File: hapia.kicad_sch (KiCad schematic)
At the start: 63 parts, among them CN1 100nf, CN2 100nf, J1 Conn_ARM_JTAG_SWD_10, J2 USB_C_Receptacle_USB2.0_16P, SW1 SW_Push, SW2 SW_Push, U1 STM32F407VET6, U11 SRV05-4HTG-D, U2 AMS1117-3.3, Y1 8mhz

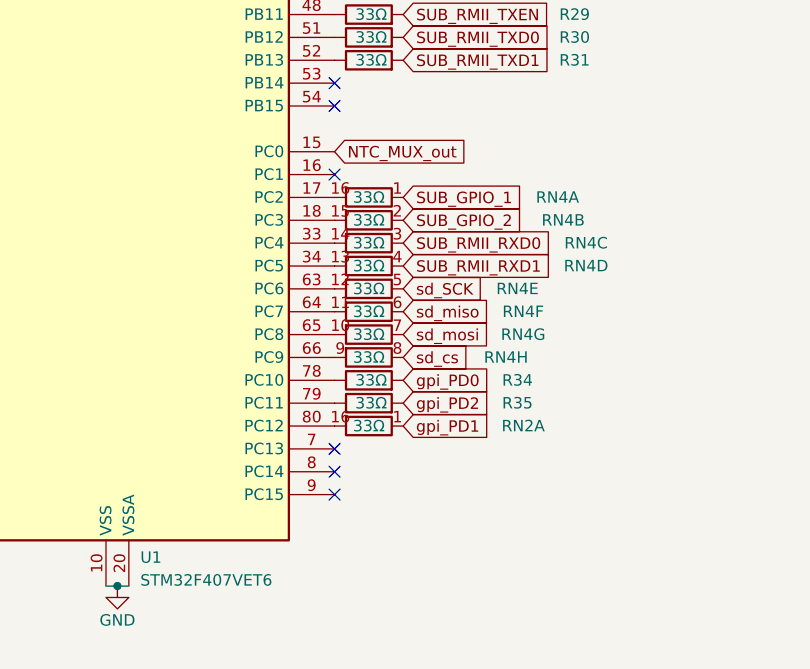
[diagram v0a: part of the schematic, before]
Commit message: 27092026/0002
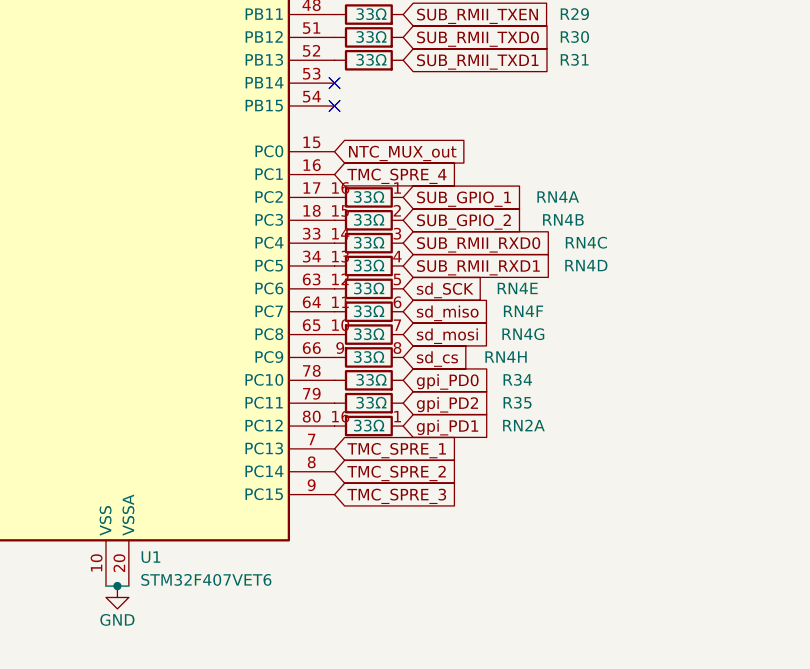
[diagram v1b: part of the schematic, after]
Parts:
- D2: footprint (none) -> LED_THT:LED_D3.0mm_FlatTop; jlc_pcb: (none) -> C7148823; mouser: (none) -> 78-VLCS5130; mpn (none) -> VLCS5130
- R1, R27: footprint (none) -> Resistor_SMD:R_0603_1608Metric Resistor_SMD_R_0603_1608Metric; jlc_pcb: (none) -> C13564; mouser: (none) -> 81-NCP18XH103F03RB; mpn (none) -> NCP18XH103F03RB
- R48: footprint (none) -> Capacitor_SMD:C_0603_1608Metric_Pad1.08x0.95mm_HandSolder; jlc_pcb: (none) -> C22548; mouser: (none) -> 603-RC0603FR-071KL; mpn (none) -> RC0603FR-071KL
- R50, R51: footprint Resistor_SMD:R_0603_1608Metric Resistor_SMD:R_0603_1608Metric -> Resistor_SMD:R_0603_1608Metric Resistor_SMD_R_0603_1608Metric
- R52: footprint (none) -> Resistor_SMD:R_0805_2012Metric_Pad1.20x1.40mm_HandSolder; jlc_pcb: (none) -> C114564; mouser: (none) -> 603-RC0805FR-07470RL; mpn (none) -> RC0805FR-07470RL
- R53, R54: footprint (none) -> Capacitor_SMD:C_0402_1005Metric_Pad0.74x0.62mm_HandSolder
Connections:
- net TMC_SPRE_4: now reaches U1.16 (PC1)
- net TMC_SPRE_1: now reaches U1.7 (PC13)
- net TMC_SPRE_2: now reaches U1.8 (PC14)
- net TMC_SPRE_3: now reaches U1.9 (PC15)
- no-connect marks 20 -> 16

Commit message: sch antigo tava jogado no pc
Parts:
- removed C6: 10µf, Capacitor_SMD:C_1206_3216Metric_Pad1.33x1.80mm_HandSolder, symbol Device:C
- removed C84: 100nf, Capacitor_SMD:C_0603_1608Metric, symbol Device:C
- removed CN1, CN2: 100nf, Capacitor_SMD:C_0603_1608Metric, symbol Device:C_Network04
- removed D2: RED, LED_THT:LED_D3.0mm_FlatTop, symbol Device:LED_Small
- removed D9: SMF3.3, Diode_SMD:D_SMF, symbol Diode:SMF5V0A
- removed F1: Fuse, symbol Device:Fuse
- removed J1: Conn_ARM_JTAG_SWD_10, symbol Connector:Conn_ARM_JTAG_SWD_10
- removed J2: USB_C_Receptacle_USB2.0_16P, Connector_USB:USB_C_Receptacle_HCTL_HC-TYPE-C-16P-01A, symbol Connector:USB_C_Receptacle_USB2.0_16P
- removed JP1: usb/atx, Jumper:SolderJumper-3_P1.3mm_Bridged2Bar12_RoundedPad1.0x1.5mm, symbol Jumper:SolderJumper_3_Bridged12
- removed R110, R111, R112, R113, R41, R42, R75: 33Ω, Resistor_SMD:R_0603_1608Metric_Pad0.98x0.95mm_HandSolder, symbol Device:R
- removed R52: 470Ω, Resistor_SMD:R_0805_2012Metric_Pad1.20x1.40mm_HandSolder, symbol Device:R_Small
- removed R54: 5.1kΩ, Capacitor_SMD:C_0402_1005Metric_Pad0.74x0.62mm_HandSolder, symbol Device:R
- removed RN2, RN4: 33Ω, Resistor_SMD:R_0603_1608Metric_Pad0.98x0.95mm_HandSolder, symbol Device:R_Pack08_Split
- removed RN5: 33Ω, Resistor_SMD:R_0603_1608Metric_Pad0.98x0.95mm_HandSolder, symbol Device:R_Pack04_Split
- removed TP1: TestPoint, TestPoint:TestPoint_Pad_D1.0mm, symbol Connector:TestPoint
- removed U11: SRV05-4HTG-D, Package_TO_SOT_SMD:SOT-23-6, symbol Power_Protection:SRV05-4
- removed U2: AMS1117-3.3, Package_TO_SOT_SMD:SOT-223-3_TabPin2, symbol Regulator_Linear:AMS1117-3.3
- added C1, C2, C21, C28, C43, C45, C59: 4.7uf, symbol Device:C
- added C13, C14, C16, C20, C23, C24, C26, C29, C34, C35, C36, C37, C39, C41, C46, C48, C53, C54, C55, C56, C58, C61, C63, C64, C65, C66, C68, C69, C70, C71: 100nf, symbol Device:C
- added C15, C25, C38, C40, C57, C62: 1uf, symbol Device:C
- added C17, C32, C33: 22nf, symbol Device:C
- added C18, C30, C47, C49, C67, C73: 10uf, symbol Device:C
- added C19, C31, C50, C51: 100uf, symbol Device:C
- added C22, C27, C42, C44, C74: 10nf, symbol Device:C
- added C52, C60: 1000uf, symbol Device:C
- added D1: D_Schottky, symbol Device:D_Schottky
- added F1, F3, F4: Polyfuse, symbol Device:Polyfuse
- added F2: Fuse, symbol Device:Fuse
- added FB2: FerriteBead, symbol Device:FerriteBead
- added J1: ATX-20, Connector_Molex:Molex_Mini-Fit_Jr_5566-20A_2x10_P4.20mm_Vertical, symbol Connector:ATX-20
- added J2: Micro_SD_Card, symbol Connector:Micro_SD_Card
- added J3, J4, J5, J6: Conn_01x04_Pin, Connector_JST:JST_EH_B4B-EH-A_1x04_P2.50mm_Vertical, symbol Connector:Conn_01x04_Pin
- added J7: Conn_01x15_Pin, Connector_PinSocket_2.54mm:PinSocket_1x15_P2.54mm_Vertical, symbol Connector:Conn_01x15_Pin
- added L1: 6.8uh, Inductor_SMD:L_Bourns_SRP1038C_10.0x10.0mm, symbol Device:L
- added M1: Fan, symbol Motor:Fan
- added Q1, Q3: NMOS, symbol Simulation_SPICE:NMOS
- added R10, R11, R12, R13, R17, R18, R19, R20, R3: 100k, symbol Device:R
- added R14, R21, R22, R9: 20k, symbol Device:R
- added R15, R16, R23, R24, R5, R6: 11r, symbol Device:R
- added R2: 10K, symbol Device:R
- added R37: 10k, symbol Device:R
- added R38: 330r, symbol Device:R
- added R39: 100r, symbol Device:R
- added R4: 22k, symbol Device:R
- added R41: exrtusora, symbol Device:Heater
- added R43, R45, R46, R47, R48, R52, R8: 33r, symbol Device:R
- added SW3: SW_Push, symbol Switch:SW_Push
- added TP3: TestPoint, Connector_USB:USB_Micro-B_Amphenol_10104110_Horizontal, symbol Connector:TestPoint
- added U2, U4, U5, U6: TMC2209-LA, Package_DFN_QFN:VQFN-28-1EP_5x5mm_P0.5mm_EP3.7x3.7mm_ThermalVias, symbol Driver_Motor:TMC2209-LA
- added U3: TPS54302, Package_TO_SOT_SMD:SOT-23-6, symbol Regulator_Switching:TPS54302
- C10: value 4.7µf -> 100nf; footprint Capacitor_SMD:C_0603_1608Metric_Pad1.08x0.95mm_HandSolder -> (none); jlc_pcb: C162274 -> (none); mouser: 81-GRM188R61E475KE1D -> (none); mpn GRM188R61E475KE11D -> (none)
- C11: value 10µf -> 100nf; footprint Capacitor_SMD:C_1206_3216Metric_Pad1.33x1.80mm_HandSolder -> (none); jlc_pcb: C13585 -> (none); mouser: 187-CL31B106KLK6PNE -> (none); mpn CL31A106KBHNNNE -> (none)
- C12: value 1µf -> 22nf; footprint Capacitor_SMD:C_0805_2012Metric_Pad1.18x1.45mm_HandSolder -> (none); jlc_pcb: C28323 -> (none); mouser: 187-CL21B105KBFNNNE -> (none); mpn CL21B105KBFNNNE -> (none)
- C3: renamed from C5; value 22pf -> pf; footprint Capacitor_SMD:C_0603_1608Metric_Pad1.08x0.95mm_HandSolder -> (none); jlc_pcb: C561800 -> (none); mouser: 80-C0603C220J4G -> (none); mpn C0603C220J4GAC7867 -> (none)
- C4: renamed from C1; value 22pf -> pf; footprint Capacitor_SMD:C_0603_1608Metric_Pad1.08x0.95mm_HandSolder -> (none); jlc_pcb: C561800 -> (none); mouser: 80-C0603C220J4G -> (none); mpn C0603C220J4GAC7867 -> (none)
- C5: renamed from C4; footprint Capacitor_SMD:C_0603_1608Metric -> (none); jlc_pcb/lcsc_ID: C346191 -> (none); jlc_pcb: C307348 -> (none); mouser: 187-CL10B104KB8WPNC -> (none); mpn CL10B104KB8WPNC -> (none)
- C6: renamed from C3; footprint Capacitor_SMD:C_0603_1608Metric -> (none); jlc_pcb/lcsc_ID: C346191 -> (none); jlc_pcb: C307348 -> (none); mouser: 187-CL10B104KB8WPNC -> (none); mpn CL10B104KB8WPNC -> (none)
- C7: footprint Capacitor_SMD:C_0603_1608Metric -> (none); jlc_pcb/lcsc_ID: C346191 -> (none); jlc_pcb: C307348 -> (none); mouser: 187-CL10B104KB8WPNC -> (none); mpn CL10B104KB8WPNC -> (none)
- C72: renamed from C2; value 10µf -> 10uf; footprint Capacitor_SMD:C_1206_3216Metric_Pad1.33x1.80mm_HandSolder -> (none); jlc_pcb: C13585 -> (none); mouser: 187-CL31B106KLK6PNE -> (none); mpn CL31A106KBHNNNE -> (none)
- C8: value 4.7µf -> 10uf; footprint Capacitor_SMD:C_0603_1608Metric_Pad1.08x0.95mm_HandSolder -> (none); Descrição capacitor ceramico 4.7uf(µf) -> (none); jlc_pcb: C162274 -> (none); mouser: 81-GRM188R61E475KE1D -> (none); mpn GRM188R61E475KE11D -> (none)
- C9: value 100nf -> 10uf; footprint Capacitor_SMD:C_0603_1608Metric -> (none); jlc_pcb/lcsc_ID: C346191 -> (none); jlc_pcb: C307348 -> (none); mouser: 187-CL10B104KB8WPNC -> (none); mpn CL10B104KB8WPNC -> (none)
- R1: value 10KΩ -> 10K; footprint Resistor_SMD:R_0603_1608Metric Resistor_SMD_R_0603_1608Metric -> (none); jlc_pcb: C13564 -> (none); mouser: 81-NCP18XH103F03RB -> (none); mpn NCP18XH103F03RB -> (none)
- R25, R26: value 22Ω -> 11r; footprint Resistor_SMD:R_0603_1608Metric_Pad0.98x0.95mm_HandSolder -> (none); jlc_pcb: C71618 -> (none); mouser: 71-CRCW0603-22-E3 -> (none); mpn CRCW060322R0FKEA -> (none)
- R27: value 10KΩ -> 1k; footprint Resistor_SMD:R_0603_1608Metric Resistor_SMD_R_0603_1608Metric -> (none); jlc_pcb: C13564 -> (none); mouser: 81-NCP18XH103F03RB -> (none); mpn NCP18XH103F03RB -> (none)
- R28, R30, R32, R33, R34, R35, R36, R49: value 33Ω -> 33r; footprint Resistor_SMD:R_0603_1608Metric_Pad0.98x0.95mm_HandSolder -> (none); jlc_pcb: C71618 -> (none); mouser: 71-CRCW0603-22-E3 -> (none); mpn CRCW060322R0FKEA -> (none)
- R29, R31: value 33Ω -> 1k; footprint Resistor_SMD:R_0603_1608Metric_Pad0.98x0.95mm_HandSolder -> (none); jlc_pcb: C71618 -> (none); mouser: 71-CRCW0603-22-E3 -> (none); mpn CRCW060322R0FKEA -> (none)
- R40: value 33Ω -> 10k; footprint Resistor_SMD:R_0603_1608Metric_Pad0.98x0.95mm_HandSolder -> (none); jlc_pcb: C71618 -> (none); mouser: 71-CRCW0603-22-E3 -> (none); mpn CRCW060322R0FKEA -> (none)
- R50, R51: value 10kΩ -> 33r; footprint Resistor_SMD:R_0603_1608Metric Resistor_SMD_R_0603_1608Metric -> (none); jlc_pcb: C13564 -> (none); mouser: 81-NCP18XH103F03RB -> (none); mpn NCP18XH103F03RB -> (none)
- R53: value 5.1kΩ -> 33r; footprint Capacitor_SMD:C_0402_1005Metric_Pad0.74x0.62mm_HandSolder -> (none); jlc_pcb: C105872 -> (none); mouser: 603-RC0402FR-075K1L -> (none); mpn RC0402FR-075K1L -> (none)
- R7: renamed from R48; value 1kΩ -> 1k; footprint Capacitor_SMD:C_0603_1608Metric_Pad1.08x0.95mm_HandSolder -> (none); jlc_pcb: C22548 -> (none); mouser: 603-RC0603FR-071KL -> (none); mpn RC0603FR-071KL -> (none)
- SW1: renamed from SW2; footprint Connector_PinHeader_2.54mm:PinHeader_1x02_P2.54mm_Vertical -> (none); jlc_pcb: C234182 -> (none); mouser: 538-22-28-4020 -> (none); mpn 22284020 -> (none)
- SW2: renamed from SW1; footprint Connector_PinHeader_2.54mm:PinHeader_1x02_P2.54mm_Vertical -> (none); jlc_pcb: C234182 -> (none); mouser: 538-22-28-4020 -> (none); mpn 22284020 -> (none)
- TP1: renamed from TP3; value 3.3v -> TestPoint; footprint TestPoint:TestPoint_Pad_D1.0mm -> Connector_USB:USB_Micro-B_Amphenol_10104110_Horizontal; now in the parts list
- TP2, TP4: footprint TestPoint:TestPoint_Pad_D1.0mm -> Connector_USB:USB_Micro-B_Amphenol_10104110_Horizontal; now in the parts list
- U1: value STM32F407VET6 -> STM32F407VETx; jlc_pcb: C28730 -> (none); mouser: 511-STM32F407VET6 -> (none); mpn STM32F407VET6 -> (none)
- Y1: value 8mhz -> Crystal; footprint Crystal:Crystal_SMD_5032-2Pin_5.0x3.2mm_HandSoldering -> (none); jlc_pcb: C144380 -> (none); mouser: 815-ABM3-8-D2Y-T -> (none); mpn ABM3-8.000MHZ-D2Y-T -> (none)
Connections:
- net SDW_SWDIO is gone; now on net GND: R40.2
- net SUB_RMII_CRS_DV is gone; now on an unnamed net: U1.32 (PA7)
- net SUB_RMII_TXD1 is gone; now on an unnamed net: R31.2
- net SUB_RMII_TXEN is gone; now on an unnamed net: R29.2
- net SWD_SWO is gone; now on net exrtusora: U1.35 (PB0)
- net USB_C_D+ is gone; now on net GND: R26.2
- net USB_C_D- is gone; now on net GND: R25.2
- net cc1 is gone; now on an unnamed net: R53.1
- net gpi_PD0 is gone; now on net sd_miso: R34.2
- net gpi_PD12 is gone; now on net sd_SCK: R33.2
- net gpi_PD13 is gone; now on net sd_cs: R36.2
- net gpi_PD2 is gone; now on net sd_mosi: R35.2
- net +3.3V: now also C5.1, C6.1, C72.1, FB1.2, R1.2, SW1.2, SW2.2, TP1.1, TP2.1, U1.100 (VDD), U1.11 (VDD), U1.14 (NRST), U1.19 (VDD), U1.28 (VDD), U1.50 (VDD), U1.6 (VBAT), U1.75 (VDD), U1.94 (BOOT0), C14.2, C15.2, C22.2, C23.2, C25.2, C27.2, C34.2, C36.2, C38.2, C40.2, C42.2, C44.2, C61.1, C62.1, C63.1, C64.1, C65.1, C66.1, C67.1, C68.1, C69.1, C70.1, C71.1, C73.1, C74.1, F4.2, FB2.2, J2.4 (VDD), R14.1, R2.2, R21.1, R22.1, R9.1, TP3.1, U2.15 (VCC_IO), U4.15 (VCC_IO), U5.15 (VCC_IO), U6.15 (VCC_IO)
- net GND: now also R1.1, C1.2, C13.1, C14.1, C15.1, C16.1, C18.1, C19.1, C2.2, C20.1, C21.1, C22.1, C23.1, C24.1, C25.1, C26.1, C27.1, C28.1, C29.1, C30.1, C31.1, C34.1, C35.1, C36.1, C37.1, C38.1, C39.1, C40.1, C41.1, C42.1, C43.1, C44.1, C45.1, C46.1, C47.1, C48.1, C49.1, C50.1, C51.1, C52.1, C53.1, C54.1, C55.1, C56.2, C57.2, C58.2, C59.2, C60.2, C61.2, C62.2, C63.2, C64.2, C65.2, C66.2, C67.2, C68.2, C69.2, C70.2, C71.2, C73.2, C74.2, D1.1 (K), J1.13 (GND), J1.15 (GND), J1.16 (GND), J1.17 (GND), J1.3 (GND), J1.5 (GND), J1.7 (GND), J2.6 (VSS), J2.9 (SHIELD), J7.1 (Pin_1), J7.4 (Pin_4), M1.2 (-), R10.1, R11.1, R12.1, R13.1, R15.2, R16.2, R17.1, R18.1, R19.1, R2.1, R20.1, R23.2, R24.2, R37.2, R4.2, R41.2, R5.2, R6.2, SW3.1, U2.13 (CLK), U2.18 (GND), U2.20 (STDBY), U2.29 (GND), U2.3 (GND), U3.1 (GND), U4.13 (CLK), U4.18 (GND), U4.20 (STDBY), U4.29 (GND), U4.3 (GND), U5.13 (CLK), U5.18 (GND), U5.20 (STDBY), U5.29 (GND), U5.3 (GND), U6.13 (CLK), U6.18 (GND), U6.20 (STDBY), U6.29 (GND), U6.3 (GND); no longer C12.2, C7.2, R51.2, R53.2
- net exrtusora: now also R39.1; no longer U1.44 (PE13)
- net sd_SCK: now also J2.5 (CLK)
- net sd_cs: now also J2.2 (DAT3/CD)
- net sd_miso: now also J2.7 (DAT0)
- net sd_mosi: now also J2.3 (CMD)
- net at R29.1: now also U1.29 (PA4); no longer U1.48 (PB11)
- net at U1.83 (PD2): now also R51.1
- net at R30.1: now also U1.30 (PA5); no longer U1.51 (PB12)
- net +12V: now reaches TP4.1
- net +12V: now also C16.2, C18.2, C19.2, C29.2, C30.2, C31.2, C46.2, C47.2, C48.2, C49.2, C50.2, C51.2, C52.2, C53.2, C54.2, C58.1, C59.1, C60.1, F2.2, F3.2, J7.15 (Pin_15), Q1.1 (D), Q3.1 (D), U2.22 (VS), U2.28 (VS), U4.22 (VS), U4.28 (VS), U5.22 (VS), U5.28 (VS), U6.22 (VS), U6.28 (VS)
- net at R28.1: now also R27.2, U1.26 (PA3); no longer U1.88 (PD7)
- net at U1.87 (PD6): now also R47.1
- net at R7.1: now also U1.23 (PA0); no longer U1.24 (PA1)
- net at U1.25 (PA2): now also R27.1
- net at U1.31 (PA6): now also R31.1
- net at U1.33 (PC4): now also R43.1
- net at U1.34 (PC5): now also R45.1
- net at U1.52 (PB13): no longer R31.1
- net at R25.1: now also U5.23 (BRA); no longer U1.61 (PD14)
- net at R26.1: now also U6.23 (BRA); no longer U1.62 (PD15)
- net at U1.72 (PA13): no longer R40.1
- net at C10.1, C9.1: now also FB1.1, L1.2, R3.1; no longer U1.73 (VCAP_2)
- net at U1.77 (PA15): now also R36.1
- net at U1.78 (PC10): now also R33.1; no longer R34.1
- net at R35.1: now also U1.80 (PC12); no longer U1.79 (PC11)
- net at U1.82 (PD1): now also R52.1
- net at U1.84 (PD3): now also R50.1
- net at U1.85 (PD4): now also R49.1
- net at U1.86 (PD5): now also R48.1
- net at R32.1: no longer U1.89 (PB3)
- net at U1.90 (PB4): no longer R33.1
- net at U1.91 (PB5): no longer R36.1
- net +3.3Vdev: no longer names the net of C12.1
- net +3.3Vdev: now also U2.4 (CPO)
- net +5Vusb: no longer names the net of C11.1
- net +5Vusb: now also C8.1, F3.1, U3.3 (VIN); no longer R50.1
- removed net 3.3v/1: C72.1, FB1.2, R1.2, R27.2, TP1.1, U1.100 (VDD), U1.11 (VDD), U1.19 (VDD), U1.28 (VDD), U1.50 (VDD), U1.6 (VBAT), U1.75 (VDD)
- net ATX_PWR_o: no longer names the net of U1.97 (PE0)
- net Fan_1: no longer names the net of U1.46 (PE15)
- net Fan_2: no longer names the net of U1.43 (PE12)
- net MUX_EN: no longer names the net of U1.98 (PE1)
- net NTC_MUX_0: no longer names the net of U1.3 (PE4)
- net NTC_MUX_1: no longer names the net of U1.4 (PE5)
- net NTC_MUX_2: no longer names the net of U1.5 (PE6)
- net NTC_MUX_out: no longer names the net of U1.15 (PC0)
- removed net STM_boot: C5.1, R1.1, SW1.2, U1.94 (BOOT0)
- removed net STM_nrst: C6.1, R27.1, SW2.2, TP2.1, U1.14 (NRST)
- net SUB_1: no longer names the net of U1.60 (PD13)
- net SUB_2: no longer names the net of U1.59 (PD12)
- net SUB_3: no longer names the net of U1.58 (PD11)
- net SUB_4: no longer names the net of U1.57 (PD10)
- net SUB_5: no longer names the net of U1.56 (PD9)
- net SUB_6: no longer names the net of U1.1 (PE2)
- net SUB_6: no longer U1.55 (PD8)
- net SUB_RMII_TXD0 renamed TMC_uart3
- net TMC_uart3: now also U4.14 (~{PD}/UART)
- net SUB_SCL: no longer names the net of U1.92 (PB6)
- net SUB_SDA: no longer names the net of U1.93 (PB7)
- net SUB_led: no longer names the net of U1.2 (PE3)
- net SWD/jtag_rst: no longer names the net of U1.36 (PB1)
- net TMC_SPRE_1: no longer names the net of U1.7 (PC13)
- net TMC_SPRE_2: no longer names the net of U1.8 (PC14)
- net TMC_SPRE_3: no longer names the net of U1.9 (PC15)
- net TMC_SPRE_4: no longer names the net of U1.16 (PC1)
- net TMC_uart renamed gpi_5
- net gpi_5: now also J7.8 (Pin_8)
- net USB_det_2.5v renamed gpi_4
- net gpi_4: now also J7.9 (Pin_9); no longer R51.1
- removed net VDDA: FB1.1, U1.21 (VREF+), U1.22 (VDDA)
- net gpi_PD10 renamed TMC_uart2
- net TMC_uart2: now also U6.14 (~{PD}/UART)
- net gpi_PD11 renamed TMC_uart4
- net TMC_uart4: now also U5.14 (~{PD}/UART)
- net gpi_PD14: no longer names the net of U1.70 (PA11)
- net gpi_PD15: no longer names the net of U1.71 (PA12)
- net hot_bed: no longer names the net of U1.45 (PE14)
- new net: J3.1 (Pin_1), U2.1 (OB2)
- new net: R9.2, U2.2 (~{EN})
- new net: J3.3 (Pin_3), U2.21 (OA2)
- new net: R6.1, U2.23 (BRA)
- new net: J3.4 (Pin_4), U2.24 (OA1)
- new net: J3.2 (Pin_2), U2.26 (OB1)
- new net: R5.1, U2.27 (BRB)
- new net: C12.2, U2.5 (CPI)
- new net: J5.1 (Pin_1), U5.1 (OB2)
- new net: R21.2, U5.2 (~{EN})
- new net: J5.3 (Pin_3), U5.21 (OA2)
- new net: J5.4 (Pin_4), U5.24 (OA1)
- new net: J5.2 (Pin_2), U5.26 (OB1)
- new net: R23.1, U5.27 (BRB)
- new net: C32.1, U5.4 (CPO)
- new net: C32.2, U5.5 (CPI)
- new net: C1.1, U1.73 (VCAP_2)
- new net: F4.1, J7.14 (Pin_14)
- new net: J6.1 (Pin_1), U6.1 (OB2)
- new net: R22.2, U6.2 (~{EN})
- new net: J6.3 (Pin_3), U6.21 (OA2)
- new net: J6.4 (Pin_4), U6.24 (OA1)
- new net: J6.2 (Pin_2), U6.26 (OB1)
- new net: R24.1, U6.27 (BRB)
- new net: C33.1, U6.4 (CPO)
- new net: C33.2, U6.5 (CPI)
- new net: C55.2, D1.2 (A), M1.1 (+), Q1.3 (S)
- new net: C2.1, U1.49 (VCAP_1)
- new net: R7.2, R8.1, U1.24 (PA1)
- new net: FB2.1, U1.22 (VDDA)
- new net: R34.1, U1.79 (PC11)
- new net: R46.1, U1.88 (PD7)
- new net: Q3.2 (G), R39.2, R40.1
- new net: C17.1, U4.4 (CPO)
- new net: C17.2, U4.5 (CPI)
- new net: R3.2, R4.1, U3.4 (FB)
- new net: C7.1, U3.6 (BOOT)
- new net: C7.2, L1.1, U3.2 (SW)
- new net: Q3.3 (S), R41.1
- new net: Q1.2 (G), R37.1, R38.2
- new net: R14.2, U4.2 (~{EN})
- new net: F1.1, J1.19 (+5V), J1.20 (+5V), J1.4 (+5V), J1.6 (+5V)
- new net: R16.1, U4.23 (BRA)
- new net: J4.1 (Pin_1), U4.1 (OB2)
- new net: J4.3 (Pin_3), U4.21 (OA2)
- new net: J4.4 (Pin_4), U4.24 (OA1)
- new net: J4.2 (Pin_2), U4.26 (OB1)
- new net: R15.1, U4.27 (BRB)
- new net: J1.1 (+3.3V), J1.11 (+3.3V), J1.2 (+3.3V)
- new net: F2.1, J1.10 (+12V)
- new net +5V: C56.1, C57.1, F1.2, J7.13 (Pin_13)
- new net 3.3v/A: U1.21 (VREF+)
- new net ATX_on: J1.14 (PS_ON#), SW3.2
- new net STM_ADC: J7.2 (Pin_2), R43.2
- new net STM_ADC_1: J7.3 (Pin_3), R45.2
- new net TMC_1vcp: C13.2, U2.6 (VCP)
- new net TMC_1vut: C20.2, C21.2, U2.8 (5VOUT)
- new net TMC_2vcp: C37.2, U6.6 (VCP)
- new net TMC_2vut: C41.2, U6.8 (5VOUT)
- new net TMC_3vcp: C24.2, U4.6 (VCP)
- new net TMC_3vut: C26.2, C28.2, U4.8 (5VOUT)
- new net TMC_4vcp: C35.2, U5.6 (VCP)
- new net TMC_4vut: C43.2, U5.8 (5VOUT)
- new net TMC_MS1_1: R11.2, R20.2, U2.9 (MS1/AD0)
- new net TMC_MS1_2: R10.2, R18.2, U2.10 (MS2/AD1), U6.9 (MS1/AD0)
- new net TMC_MS1_3: R13.2, U4.9 (MS1/AD0)
- new net TMC_MS1_4: R19.2, U5.9 (MS1/AD0)
- new net TMC_MS2_2: U6.10 (MS2/AD1)
- new net TMC_MS2_3: R12.2, U4.10 (MS2/AD1)
- new net TMC_MS2_4: R17.2, U5.10 (MS2/AD1)
- new net TMC_uart1: R8.2, U2.14 (~{PD}/UART)
- new net gpi_1: J7.12 (Pin_12), R53.2
- new net gpi_2: J7.11 (Pin_11), R52.2
- new net gpi_3: J7.10 (Pin_10), R51.2
- new net gpi_6: J7.7 (Pin_7), R48.2
- new net gpi_7: J7.6 (Pin_6), R47.2
- new net gpi_8: J7.5 (Pin_5), R46.2
- no-connect marks 16 -> 33
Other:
- note removed: "3.3vbus = usb, 3.3v = atx"
- note removed: "Q1"
- note removed: "Q1: o pino "shield" ta em "nc" por que essa impresora vai ser um "slave"/device, com modificação funciona com pendrive."
- note removed: "Q2"
- note removed: "by todio"
- note removed: "ele ja vem com alimentaçao por usb"
- note removed: "se o mcu não tiver ligando com usb possivelmente o problema e o jumper(o pino do meio) não ligado a o pino de cima o 3.3vdev ou fusivel queimado. se esse não for o defeito provavelmente e algum componente com defeito."
- company: --- -> (none)
- title: hapia placa base. -> (none)
- moved on the sheet: C3, C4, C5, C6, C72, R7, SW1, SW2, TP1, U1, Y1
